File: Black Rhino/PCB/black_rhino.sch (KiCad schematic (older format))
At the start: 174 parts, among them SW1 SW_Push, U1 ATmega32U4-AU, Y1 16MHz

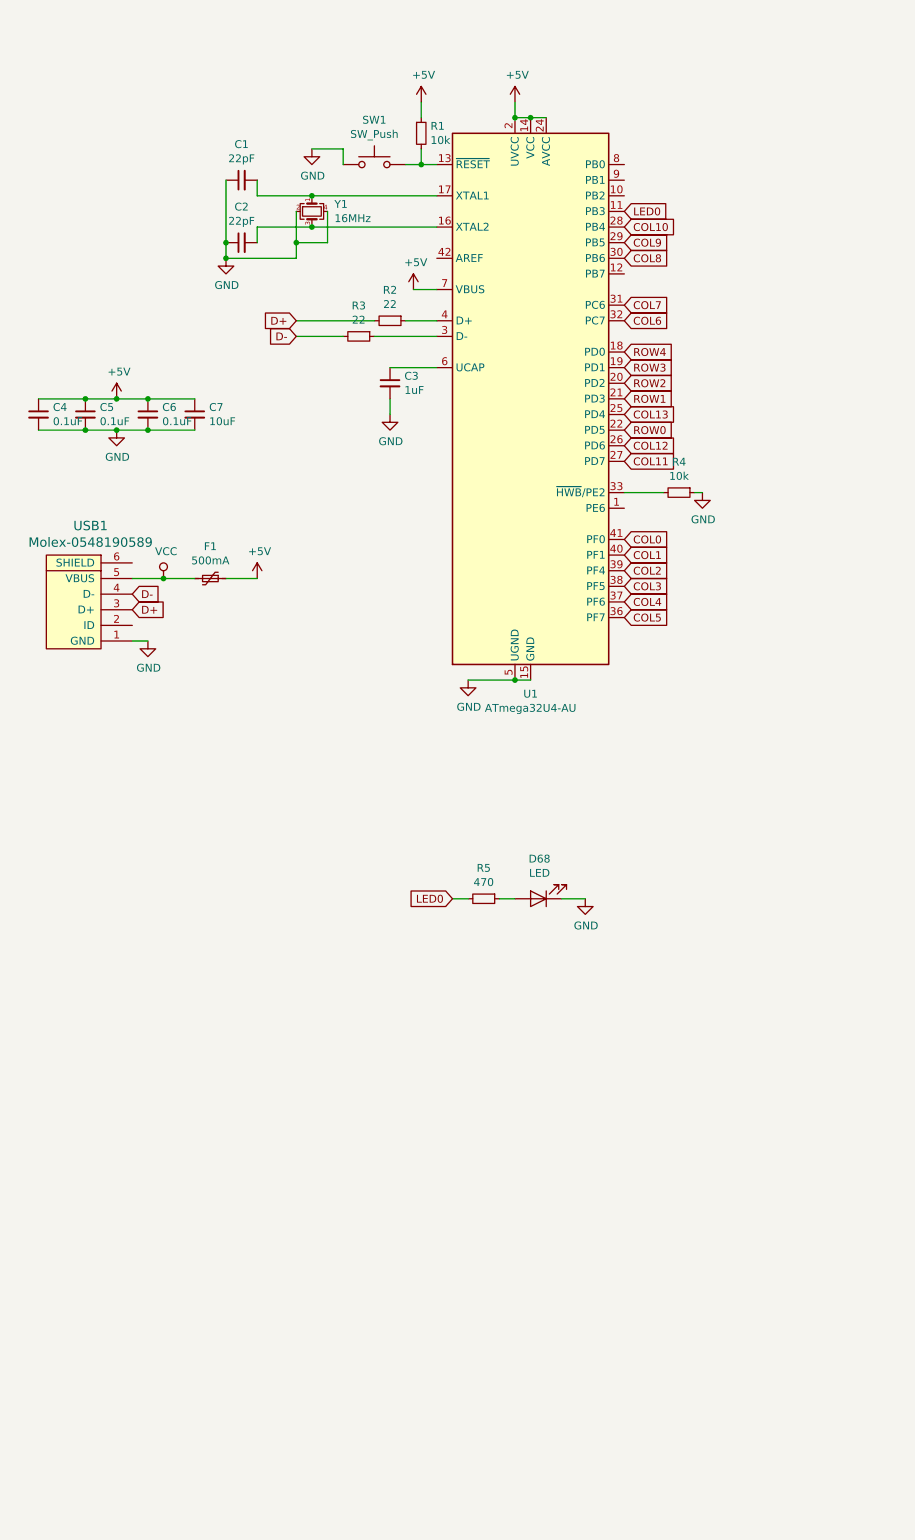
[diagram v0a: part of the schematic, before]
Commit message: Improve Black Rhino-PCB
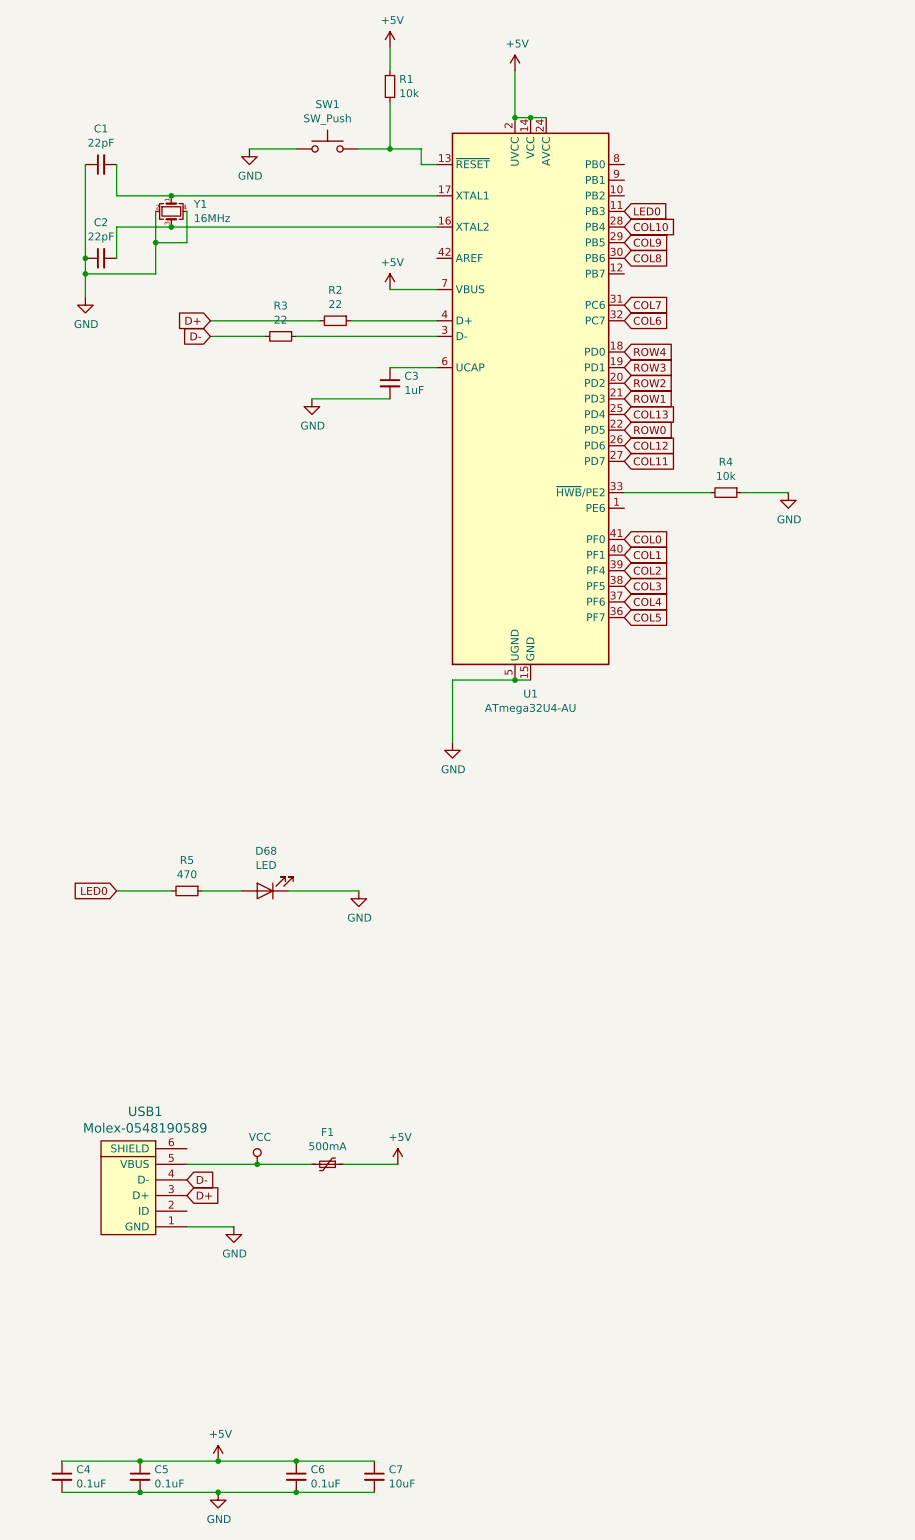
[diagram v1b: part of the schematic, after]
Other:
- moved on the sheet: C1, C2, C4, C5, C6, C7, D68, F1, R1, R2, R3, R4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
